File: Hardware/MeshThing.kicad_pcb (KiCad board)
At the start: 2 copper layers, 25.7 x 27.8 mm, 28 parts, among them IC1 ATMEGA2564/1284/644RFR2, SW1 RST, U1 CONN_MICROSD, U2 XBEE, U3 XBEE

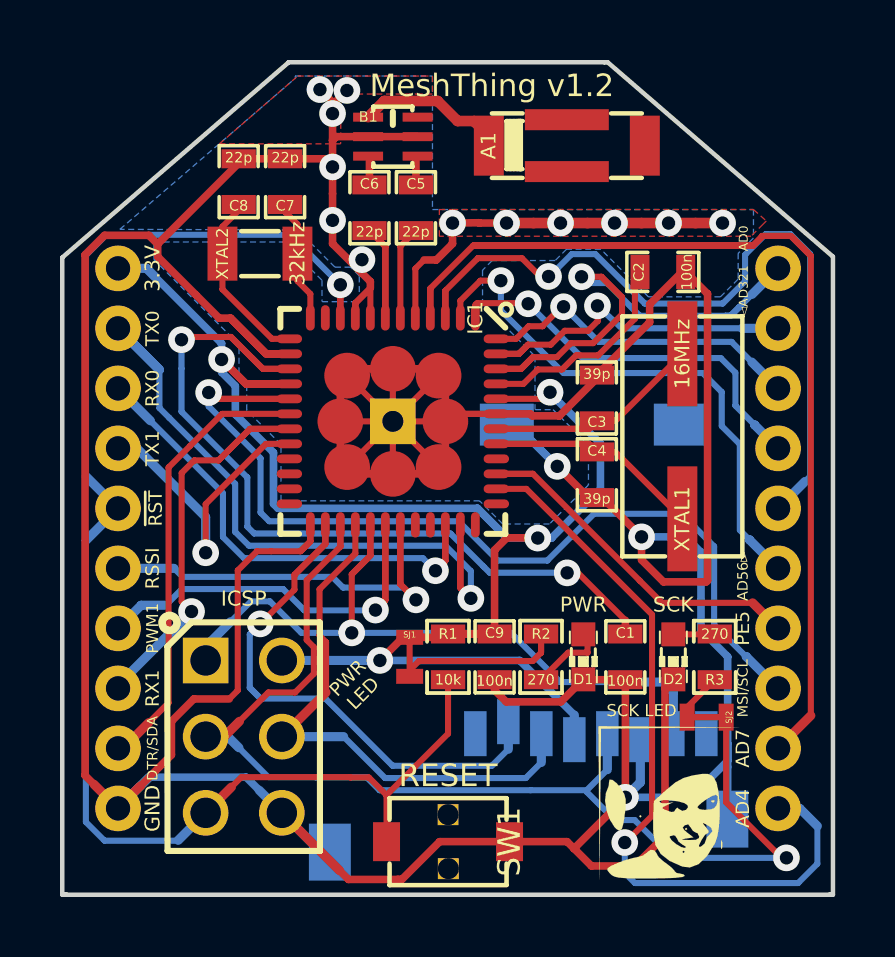
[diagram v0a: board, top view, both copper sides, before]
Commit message: More checks.
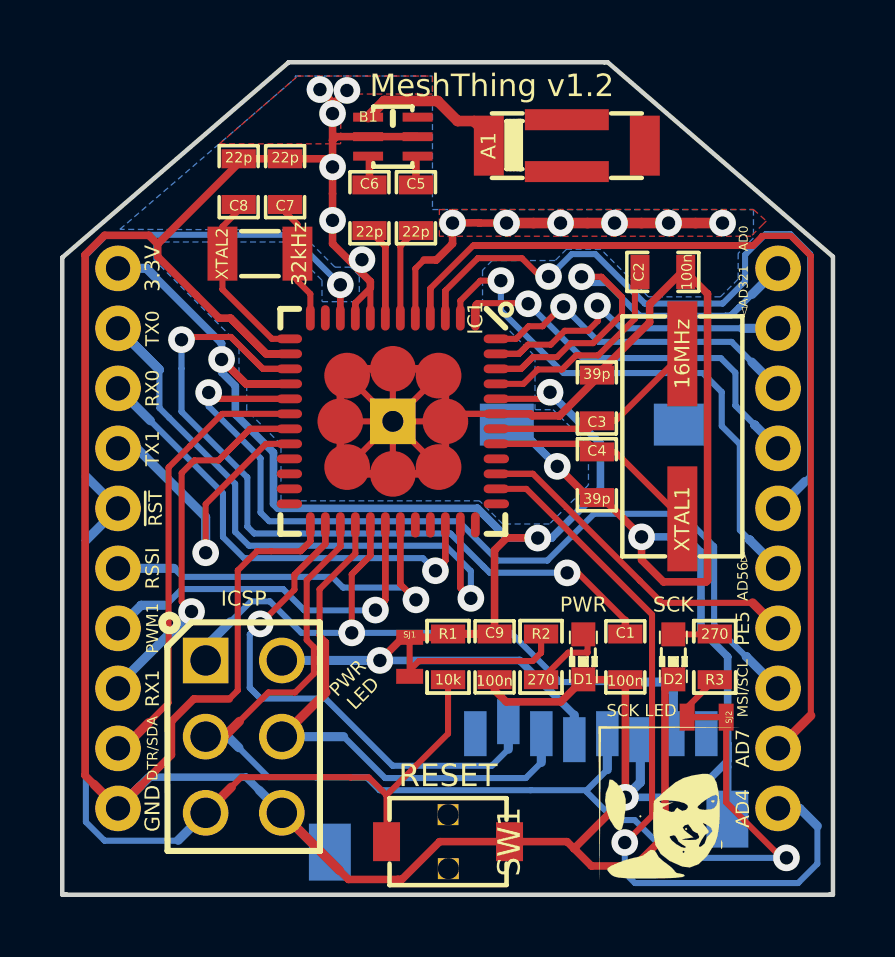
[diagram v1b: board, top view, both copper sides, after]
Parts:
- turned XTAL2 to 0 degrees
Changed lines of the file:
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@@
     (18 B.Paste user)
     (19 F.Paste user)
-    (20 B.SilkS user hide)
+    (20 B.SilkS user)
     (21 F.SilkS user)
     (22 B.Mask user)
@@
     (mod_text_size 1.5 1.5)
     (mod_text_width 0.15)
-    (pad_size 1 0.3)
+    (pad_size 0.8 0.8)
     (pad_drill 0)
     (pad_to_mask_clearance 0.2)
     (pad_to_paste_clearance_ratio -0.1)
     (aux_axis_origin 135.66 132.51)
-    (visible_elements FFFFFF7F)
+    (visible_elements FFFFF77F)
     (pcbplotparams
       (layerselection 284983297)
@@
       (xy -1.36398 2.0193)) (layer B.SilkS) (width 0.00254))
   )
-  (module _MT_TF32D-32768-Crystal (layer F.Cu)
-    (at 142.37 110.9 180)
-    (fp_text reference XTAL2 (at 1.25 0 270) (layer F.SilkS)
-      (effects (font (size 0.4 0.4) (thickness 0.1)))
-    )
-    (fp_text value 32kHz (at -1.25 0 270) (layer F.SilkS)
-      (effects (font (size 0.5 0.5) (thickness 0.125)))
-    )
-    (fp_line (start -0.625 -0.75) (end 0.625 -0.75) (layer F.SilkS) (width 0.15))
-    (fp_line (start -0.625 0.75) (end 0.625 0.75) (layer F.SilkS) (width 0.15))
-    (pad 1 smd rect (at 1.25 0 180) (size 1 1.8)
-      (layers F.Cu F.Paste F.Mask)
-      (net 15 N-0000027)
-    )
-    (pad 2 smd rect (at -1.25 0 180) (size 1 1.8)
-      (layers F.Cu F.Paste F.Mask)
-      (net 16 N-0000028)
-    )
-  )
   (module _MT_LED-0603 (layer F.Cu)
     (at 156.15 124.34 90)
@@
       (layers F.Cu F.Paste F.Mask)
       (net 31 N-0000056)
+    )
+  )
+  (module _MT_TF32D-32768-Crystal (layer F.Cu)
+    (at 142.37 110.9)
+    (fp_text reference XTAL2 (at -1.26 0 90) (layer F.SilkS)
+      (effects (font (size 0.4 0.4) (thickness 0.1)))
+    )
+    (fp_text value 32kHz (at 1.31 0.01 90) (layer F.SilkS)
+      (effects (font (size 0.5 0.5) (thickness 0.125)))
+    )
+    (fp_line (start -0.625 -0.75) (end 0.625 -0.75) (layer F.SilkS) (width 0.15))
+    (fp_line (start -0.625 0.75) (end 0.625 0.75) (layer F.SilkS) (width 0.15))
+    (pad 2 smd rect (at 1.25 0) (size 1 1.8)
+      (layers F.Cu F.Paste F.Mask)
+      (net 16 N-0000028)
+    )
+    (pad 1 smd rect (at -1.25 0) (size 1 1.8)
+      (layers F.Cu F.Paste F.Mask)
+      (net 15 N-0000027)
     )
   )
@@
   (segment (start 156.61 126.022) (end 157.53 125.102) (width 0.2032) (layer F.Cu) (net 14))
   (segment (start 141.66 109.262) (end 141.66 109.46) (width 0.2032) (layer F.Cu) (net 15))
+  (segment (start 143.35068 113.74) (end 142.77 113.74) (width 0.2032) (layer F.Cu) (net 15))
+  (segment (start 142.77 113.74) (end 141.12 112.09) (width 0.2032) (layer F.Cu) (net 15))
   (segment (start 141.12 110) (end 141.12 110.9) (width 0.2032) (layer F.Cu) (net 15))
   (segment (start 141.66 109.46) (end 141.12 110) (width 0.2032) (layer F.Cu) (net 15))
-  (segment (start 143.35068 113.74) (end 142.77 113.74) (width 0.2032) (layer F.Cu) (net 15))
-  (segment (start 142.77 113.74) (end 141.12 112.09) (width 0.2032) (layer F.Cu) (net 15))
   (segment (start 141.12 112.09) (end 141.12 110.9) (width 0.2032) (layer F.Cu) (net 15))
+  (segment (start 143.62 109.92) (end 143.62 110.9) (width 0.2032) (layer F.Cu) (net 16))
+  (segment (start 143.62 111.81055) (end 143.62 110.9) (width 0.2032) (layer F.Cu) (net 16))
   (segment (start 143.21 109.262) (end 143.21 109.51) (width 0.2032) (layer F.Cu) (net 16))
-  (segment (start 143.62 109.92) (end 143.62 110.9) (width 0.2032) (layer F.Cu) (net 16))
   (segment (start 143.21 109.51) (end 143.62 109.92) (width 0.2032) (layer F.Cu) (net 16))
+  (segment (start 144.05 112.24055) (end 143.62 111.81055) (width 0.2032) (layer F.Cu) (net 16))
   (segment (start 144.05 113.04068) (end 144.05 112.24055) (width 0.2032) (layer F.Cu) (net 16))
-  (segment (start 143.62 111.81055) (end 143.62 110.9) (width 0.2032) (layer F.Cu) (net 16))
-  (segment (start 144.05 112.24055) (end 143.62 111.81055) (width 0.2032) (layer F.Cu) (net 16))
   (segment (start 150.24932 116.74) (end 153.332 116.74) (width 0.2032) (layer F.Cu) (net 27))
   (segment (start 153.332 116.74) (end 153.6 116.472) (width 0.2032) (layer F.Cu) (net 27))
